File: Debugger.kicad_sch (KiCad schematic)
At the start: 24 parts, among them J1 Internal clock, J2 I/O, J3 NAND0, J4 NAND1, Q1 BC546, SW1 Single step, U1 NE555P, U2 74LS132, U3 74LS74

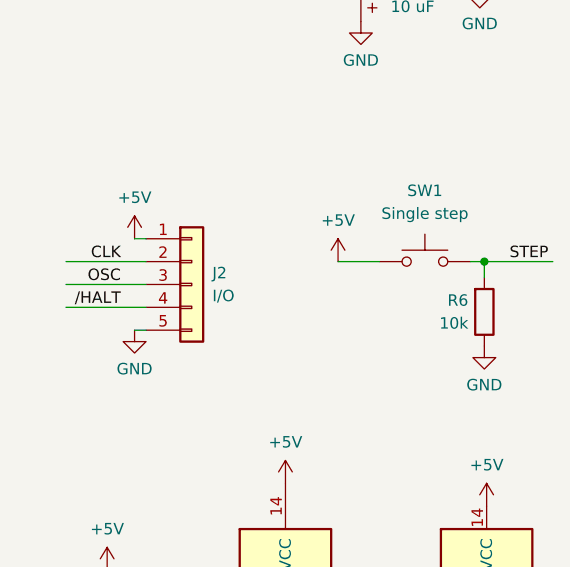
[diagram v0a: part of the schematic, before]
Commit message: Schematic: fix power flag
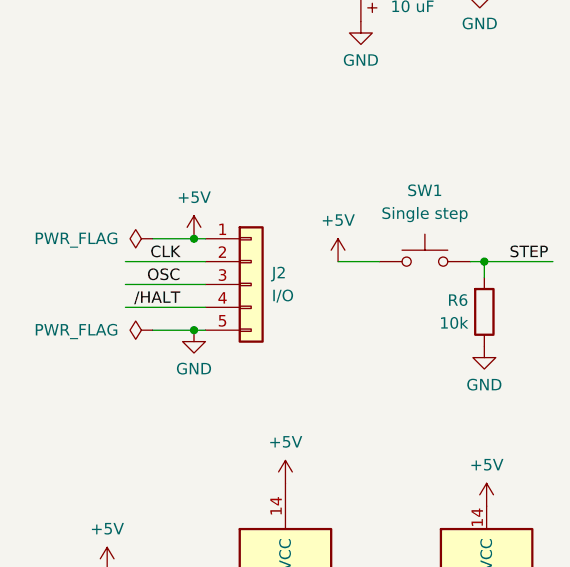
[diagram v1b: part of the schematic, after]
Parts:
- added unit 3 of U2
- added unit 5 of U2
- added unit 4 of U2
- added unit 1 of U2
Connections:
- net +5V: now also U2.14 (VCC); no longer U2.14 (VCC)
- net GND: now also U2.7 (GND); no longer U2.7 (GND)
- net at U3.9 (Q): now also U2.1; no longer U2.1
- net at J3.3 (Pin_3): now also U2.10; no longer U2.10
- net at J4.2 (Pin_2): now also U2.11; no longer U2.11
- net at J4.4 (Pin_4): now also U2.12; no longer U2.12
- net at J4.3 (Pin_3): now also U2.13; no longer U2.13
- net at U3.5 (Q): now also U2.2; no longer U2.2
- net at R3.1: now also U2.3; no longer U2.3
- net at J3.2 (Pin_2): now also U2.8; no longer U2.8
- net at J3.4 (Pin_4): now also U2.9; no longer U2.9
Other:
- moved on the sheet: J2
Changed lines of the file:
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@@
 	)
 	(junction
+		(at 34.544 85.852)
+		(diameter 0)
+		(color 0 0 0 0)
+	)
+	(junction
+		(at 34.544 75.692)
+		(diameter 0)
+		(color 0 0 0 0)
+	)
+	(junction
 		(at 82.55 27.178)
 		(diameter 0)
@@
 	(wire
 		(pts
-			(xy 27.94 75.692) (xy 29.21 75.692)
+			(xy 34.544 75.692) (xy 35.814 75.692)
 		)
 		(stroke
@@
 	(wire
 		(pts
+			(xy 29.972 85.852) (xy 34.544 85.852)
+		)
+		(stroke
+			(width 0)
+			(type default)
+		)
+	)
+	(wire
+		(pts
 			(xy 125.73 89.916) (xy 147.828 89.916)
 		)
@@
 	(wire
 		(pts
+			(xy 29.972 75.692) (xy 34.544 75.692)
+		)
+		(stroke
+			(width 0)
+			(type default)
+		)
+	)
+	(wire
+		(pts
 			(xy 133.096 39.878) (xy 135.636 39.878)
 		)
@@
 	(wire
 		(pts
-			(xy 20.32 78.232) (xy 29.21 78.232)
+			(xy 26.924 78.232) (xy 35.814 78.232)
 		)
 		(stroke
@@
 	(wire
 		(pts
-			(xy 20.32 80.772) (xy 29.21 80.772)
+			(xy 26.924 80.772) (xy 35.814 80.772)
 		)
 		(stroke
@@
 	(wire
 		(pts
-			(xy 27.94 85.852) (xy 29.21 85.852)
+			(xy 34.544 85.852) (xy 35.814 85.852)
 		)
 		(stroke
@@
 	(wire
 		(pts
-			(xy 20.32 83.312) (xy 29.21 83.312)
+			(xy 26.924 83.312) (xy 35.814 83.312)
 		)
 		(stroke
@@
 	)
 	(label "OSC"
-		(at 26.416 80.772 180)
+		(at 33.02 80.772 180)
 		(effects
 			(font
@@
 	)
 	(label "{slash}HALT"
-		(at 26.416 83.312 180)
+		(at 33.02 83.312 180)
 		(effects
 			(font
@@
 	)
 	(label "CLK"
-		(at 26.416 78.232 180)
+		(at 33.02 78.232 180)
 		(effects
 			(font
@@
 	(symbol
 		(lib_id "power:GND")
-		(at 27.94 85.852 0)
+		(at 34.544 85.852 0)
 		(unit 1)
 		(body_style 1)
@@
 		(fields_autoplaced yes)
 		(property "Reference" "#PWR021"
-			(at 27.94 92.202 0)
+			(at 34.544 92.202 0)
 			(hide yes)
 			(show_name no)
@@
 		)
 		(property "Value" "GND"
-			(at 27.94 90.17 0)
+			(at 34.544 90.17 0)
 			(show_name no)
 			(do_not_autoplace no)
@@
 		)
 		(property "Footprint" ""
-			(at 27.94 85.852 0)
+			(at 34.544 85.852 0)
 			(hide yes)
 			(show_name no)
@@
 		)
 		(property "Datasheet" ""
-			(at 27.94 85.852 0)
+			(at 34.544 85.852 0)
 			(hide yes)
 			(show_name no)
@@
 		)
 		(property "Description" "Power symbol creates a global label with name \"GND\" , ground"
-			(at 27.94 85.852 0)
+			(at 34.544 85.852 0)
 			(hide yes)
 			(show_name no)
@@
 	(symbol
 		(lib_id "Connector_Generic:Conn_01x05")
-		(at 34.29 80.772 0)
+		(at 40.894 80.772 0)
 		(unit 1)
 		(body_style 1)
@@
 		(fields_autoplaced yes)
 		(property "Reference" "J2"
-			(at 36.576 79.5019 0)
+			(at 43.18 79.5019 0)
 			(show_name no)
 			(do_not_autoplace no)
@@
 		)
 		(property "Value" "I/O"
-			(at 36.576 82.0419 0)
+			(at 43.18 82.0419 0)
 			(show_name no)
 			(do_not_autoplace no)
@@
 		)
 		(property "Footprint" "Connector_PinHeader_1.00mm:PinHeader_1x05_P1.00mm_Vertical"
-			(at 34.29 80.772 0)
+			(at 40.894 80.772 0)
 			(hide yes)
 			(show_name no)
@@
 		)
 		(property "Datasheet" ""
-			(at 34.29 80.772 0)
+			(at 40.894 80.772 0)
 			(hide yes)
 			(show_name no)
@@
 		)
 		(property "Description" "Generic connector, single row, 01x05, script generated (kicad-library-utils/schlib/autogen/connector/)"
-			(at 34.29 80.772 0)
+			(at 40.894 80.772 0)
 			(hide yes)
 			(show_name no)
@@
 	(symbol
 		(lib_id "power:+5V")
-		(at 27.94 75.692 0)
+		(at 34.544 75.692 0)
 		(unit 1)
 		(body_style 1)
@@
 		(fields_autoplaced yes)
 		(property "Reference" "#PWR020"
-			(at 27.94 79.502 0)
+			(at 34.544 79.502 0)
 			(hide yes)
 			(show_name no)
@@
 		)
 		(property "Value" "+5V"
-			(at 27.94 71.12 0)
+			(at 34.544 71.12 0)
 			(show_name no)
 			(do_not_autoplace no)
@@
 		)
 		(property "Footprint" ""
-			(at 27.94 75.692 0)
+			(at 34.544 75.692 0)
 			(hide yes)
 			(show_name no)
@@
 		)
 		(property "Datasheet" ""
-			(at 27.94 75.692 0)
+			(at 34.544 75.692 0)
 			(hide yes)
 			(show_name no)
@@
 		)
 		(property "Description" "Power symbol creates a global label with name \"+5V\""
-			(at 27.94 75.692 0)
+			(at 34.544 75.692 0)
 			(hide yes)
 			(show_name no)
@@
 	)
 	(symbol
+		(lib_id "power:PWR_FLAG")
+		(at 29.972 85.852 90)
+		(unit 1)
+		(body_style 1)
+		(exclude_from_sim no)
+		(in_bom yes)
+		(on_board yes)
+		(in_pos_files yes)
+		(dnp no)
+		(fields_autoplaced yes)
+		(property "Reference" "#FLG01"
+			(at 28.067 85.852 0)
+			(hide yes)
+			(show_name no)
+			(do_not_autoplace no)
+			(effects
+				(font
+					(size 1.27 1.27)
+				)
+			)
+		)
+		(property "Value" "PWR_FLAG"
+			(at 26.162 85.8519 90)
+			(show_name no)
+			(do_not_autoplace no)
+			(effects
+				(font
+					(size 1.27 1.27)
+				)
+				(justify left)
+			)
+		)
+		(property "Footprint" ""
+			(at 29.972 85.852 0)
+			(hide yes)
+			(show_name no)
+			(do_not_autoplace no)
+			(effects
+				(font
+					(size 1.27 1.27)
+				)
+			)
+		)
+		(property "Datasheet" ""
+			(at 29.972 85.852 0)
+			(hide yes)
+			(show_name no)
+			(do_not_autoplace no)
+			(effects
+				(font
+					(size 1.27 1.27)
+				)
+			)
+		)
+		(property "Description" "Special symbol for telling ERC where power comes from"
+			(at 29.972 85.852 0)
+			(hide yes)
+			(show_name no)
+			(do_not_autoplace no)
+			(effects
+				(font
+					(size 1.27 1.27)
+				)
+			)
+		)
+		(pin "1"
+		)
+		(instances
+			(project "Debugger"
+				(path "/a8de7697-6937-4325-b328-e8937268e3c6"
+					(reference "#FLG01")
+					(unit 1)
+				)
+			)
+		)
+	)
+	(symbol
 		(lib_id "Transistor_BJT:BC546")
 		(at 168.402 37.338 0)
@@
 					(unit 1)
 				)
+			)
+		)
+	)
+	(symbol
+		(lib_id "power:PWR_FLAG")
+		(at 29.972 75.692 90)
+		(unit 1)
+		(body_style 1)
+		(exclude_from_sim no)
+		(in_bom yes)
+		(on_board yes)
+		(in_pos_files yes)
+		(dnp no)
+		(fields_autoplaced yes)
+		(property "Reference" "#FLG02"
+			(at 28.067 75.692 0)
+			(hide yes)
+			(show_name no)
+			(do_not_autoplace no)
+			(effects
+				(font
+					(size 1.27 1.27)
+				)
+			)
+		)
+		(property "Value" "PWR_FLAG"
+			(at 26.162 75.6919 90)
+			(show_name no)
+			(do_not_autoplace no)
+			(effects
+				(font
+					(size 1.27 1.27)
+				)
+				(justify left)
+			)
+		)
+		(property "Footprint" ""
+			(at 29.972 75.692 0)
+			(hide yes)
+			(show_name no)
+			(do_not_autoplace no)
+			(effects
+				(font
+					(size 1.27 1.27)
+				)
+			)
+		)
+		(property "Datasheet" ""
+			(at 29.972 75.692 0)
+			(hide yes)
+			(show_name no)
+			(do_not_autoplace no)
+			(effects
+				(font
+					(size 1.27 1.27)
+				)
+			)
+		)
+		(property "Description" "Special symbol for telling ERC where power comes from"
+			(at 29.972 75.692 0)
+			(hide yes)
+			(show_name no)
+			(do_not_autoplace no)
+			(effects
+				(font
+					(size 1.27 1.27)
+				)
+			)
+		)
+		(pin "1"
+		)
+		(instances
+			(project "Debugger"
+				(path "/a8de7697-6937-4325-b328-e8937268e3c6"
+					(reference "#FLG02")
+					(unit 1)
+				)
